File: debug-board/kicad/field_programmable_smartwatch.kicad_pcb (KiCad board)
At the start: 4 copper layers, 47 x 32 mm, 43 parts, among them IC1 BQ24040DSQR, IC2 STM32WB55CEU6, J1 GPIO Header 1, J2 DX07S016JA1R1500, J3 GPIO Header 2, J4 SWD Header, Q1 Q_PMOS_DGS, SW1 SW_Push, SW2 SW_Push, Y1 32M, Y2 32.768k

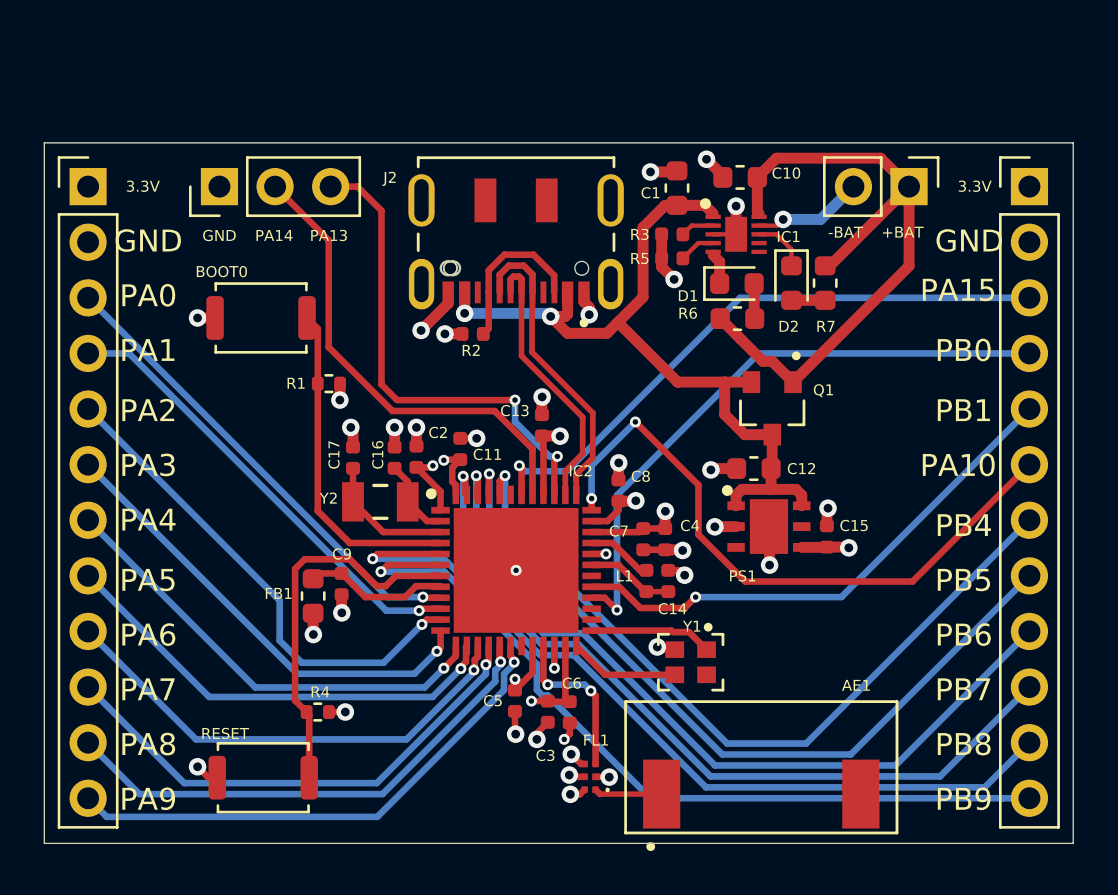
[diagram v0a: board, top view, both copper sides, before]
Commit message: Updated debug board
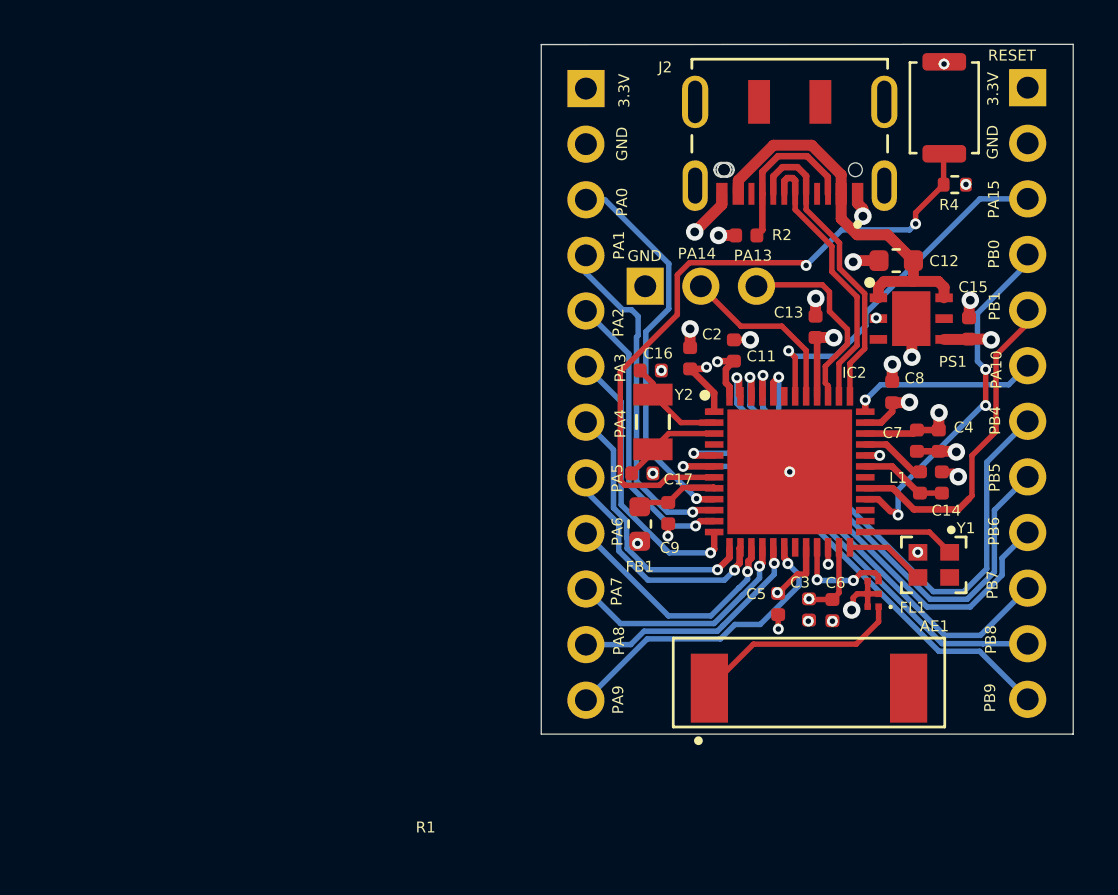
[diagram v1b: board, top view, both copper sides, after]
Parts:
- removed BT1: 3.7, Connector_PinHeader_2.54mm:PinHeader_1x02_P2.54mm_Vertical
- removed C1, C10: 1u, Capacitor_SMD:C_0603_1608Metric
- removed D1: LED_Small_Red, Diode_SMD:D_0603_1608Metric
- removed D2: LED_Small_Green, Diode_SMD:D_0603_1608Metric
- removed IC1: BQ24040DSQR, BQ2404DSQR:SON40P200X200X80-11N
- removed Q1: Q_PMOS_DGS, SSM3J325F_LF:SSM3J325F_LF
- removed R1: 100k, Resistor_SMD:R_0402_1005Metric
- removed R3: 2.87k, Resistor_SMD:R_0402_1005Metric
- removed R5: 2k, Resistor_SMD:R_0402_1005Metric
- removed R6, R7: 1.5k, Resistor_SMD:R_0603_1608Metric
- removed SW1: SW_Push, Button_Switch_SMD:SW_Push_SPST_NO_Alps_SKRK
- moved SW2 43.6 mm to (172.1, 65.4), turned to 270 degrees
- moved R4 37.8 mm to (172.6, 68.9)
- moved J1 23.2 mm to (155.7, 64.5)
- moved J4 20.0 mm to (158.4, 73.5)
- moved FL1 15.4 mm to (168.9, 87.6)
- moved FB1 15.3 mm to (158.2, 84.4)
- moved C9 15.3 mm to (159.5, 83.9)
- moved C11 13.3 mm to (162.5, 76.5)
- moved C13 13.3 mm to (166.2, 75.4)
- moved C14 13.3 mm to (172.0, 82.5)
- moved C2 13.3 mm to (160.5, 76.8)
- moved C4 13.3 mm to (171.9, 80.6)
- moved C7 13.3 mm to (170.9, 80.6)
- moved C8 13.3 mm to (169.7, 78.4)
- moved IC2 13.3 mm to (165.1, 82.0)
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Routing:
- net /+BAT: track 30.5 -> 0.00 mm
- net /PA10: track 29.4 -> 8.60 mm, vias 2 -> 1
- net GND: track 39.9 -> 19.9 mm, vias 34 -> 25
- net /VBUS: track 37.2 -> 18.1 mm, vias 2 -> 0
- net /PB8: track 38.4 -> 19.8 mm
- net /PB9: track 37.5 -> 21.6 mm
- net /BOOT0: track 15.2 -> 0.00 mm
- net /PB7: track 36.5 -> 21.3 mm
- net /PB6: track 36.8 -> 22.1 mm
- net /PA14: track 21.7 -> 8.12 mm
- net /PA13: track 22.5 -> 9.08 mm, vias 2 -> 0
- net /RESET: track 17.9 -> 30.7 mm, vias 0 -> 2
- net /PB5: track 35.6 -> 22.8 mm
- net /PA7: track 23.4 -> 10.9 mm
- net /PA8: track 23.4 -> 11.3 mm
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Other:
- board size 47 x 32 mm -> 24.3 x 31.5 mm
- board text removed: "+BAT"
- board text removed: "-BAT"
- board text removed: "BOOT0"
- board text removed: "C1"
- board text removed: "C10"
- board text removed: "D1"
- board text removed: "D2"
- board text removed: "IC1"
- board text removed: "Q1"
- board text removed: "R3"
- board text removed: "R5"
- board text removed: "R6"
- board text removed: "R7"
